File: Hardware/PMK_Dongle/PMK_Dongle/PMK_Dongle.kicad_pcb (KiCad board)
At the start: 4 copper layers, 10.4 x 18.3 mm, 32 parts, among them IC1 ESP32-S2FH4, J1 USB_A, U1 MIC5528-3.3YMT-T5, Y1 40MHz

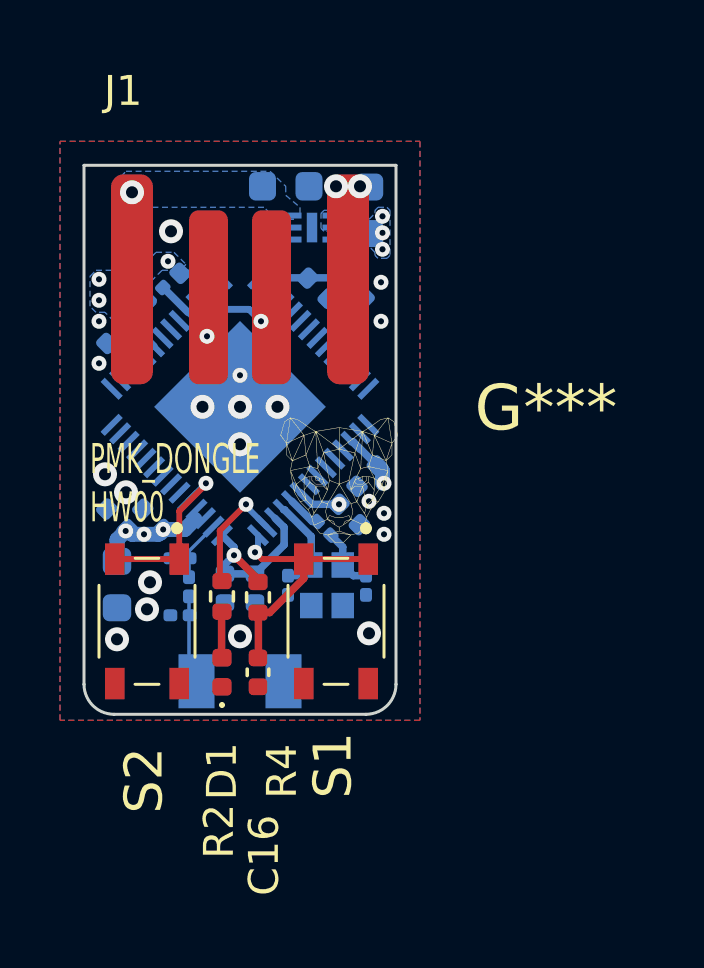
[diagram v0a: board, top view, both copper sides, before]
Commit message: Routing is done
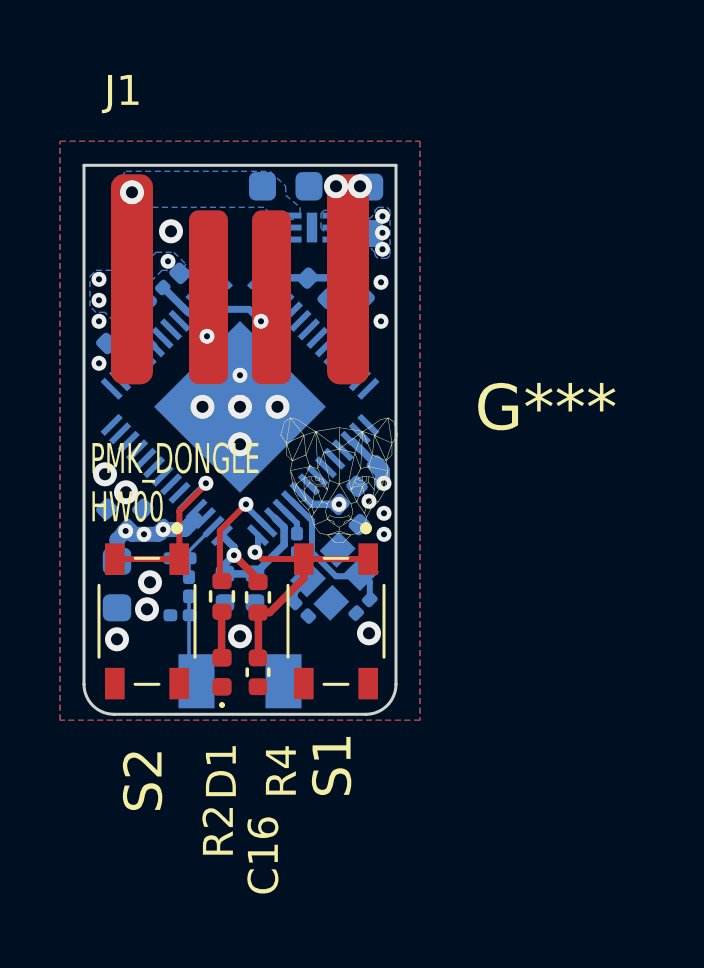
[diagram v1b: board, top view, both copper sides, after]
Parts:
- Y1: value 40MHz -> Crystal_GND24_Small; footprint Component_lib:NX2016SA32MEXS00ACS06465 -> Component_lib:Crystal_SMD_2016-4Pin_2.0x1.6mm
- moved R1 1.03 mm to (154.9, 45.8), turned to 90 degrees
- moved C3 0.92 mm to (155.1, 48.0), turned to -45 degrees
- moved C4 0.71 mm to (157.1, 47.9), turned to -135 degrees
- moved Y1 0.39 mm to (156.2, 46.9), turned to 45 degrees
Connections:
- IC1 pad 52: /QUARTZ_3 -> /QUARTZ_2
- IC1 pad 53: /QUARTZ_1 -> /QUARTZ_3
- R1 pad 1: /QUARTZ_2 -> /QUARTZ_1
- S2 pad 4: GND -> (no net)
- Y1 pad 1: /QUARTZ_2 -> /QUARTZ_1
- Y1 pad 3: GND -> /QUARTZ_2
- Y1 pad 4: /QUARTZ_1 -> GND
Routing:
- net /QUARTZ_2: track 2.09 -> 5.00 mm
- net /QUARTZ_1: track 3.17 -> 1.99 mm
